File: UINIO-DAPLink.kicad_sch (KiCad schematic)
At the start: 44 parts, among them J1 扩展板串口 & 电源输出, J2 扩展板 JTAG 输出, J3 JTAG_nTRST 跳线选择, J4 3.3V 跳线选择, J5 扩展板 SWD 输入, J6 DAPLink 固件下载接口, J7 SWD 下载输出, U1 ME6211C33M5G, U2 STM32F103C8T6, Y1 8MHz

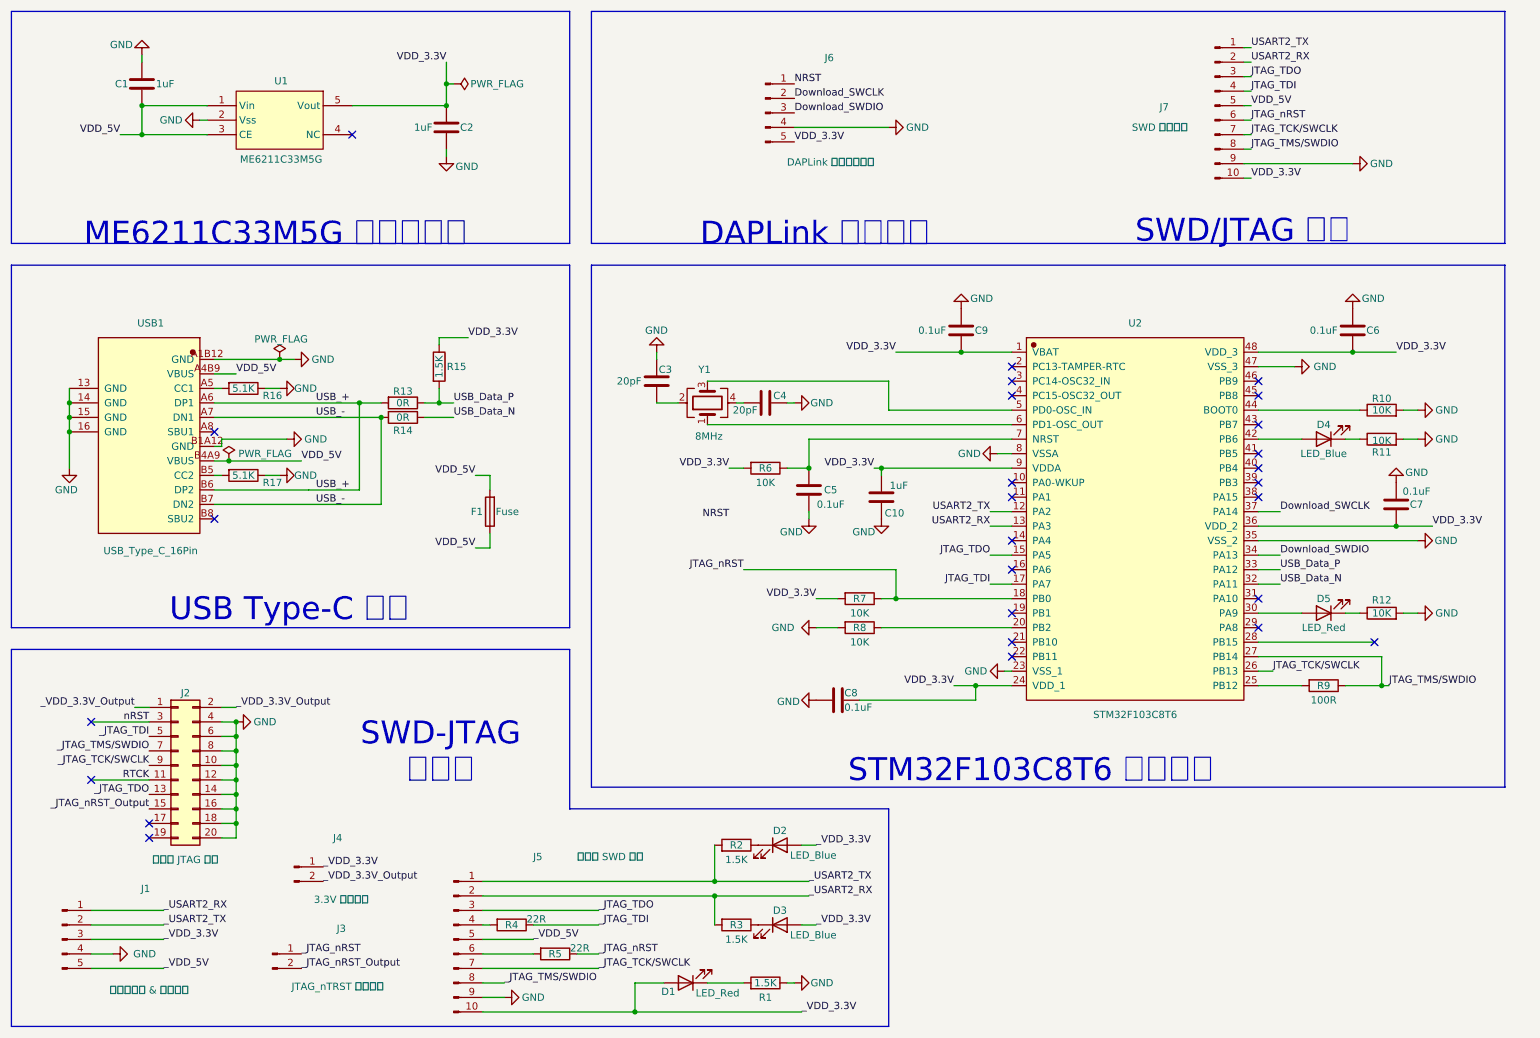
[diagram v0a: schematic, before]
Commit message: update
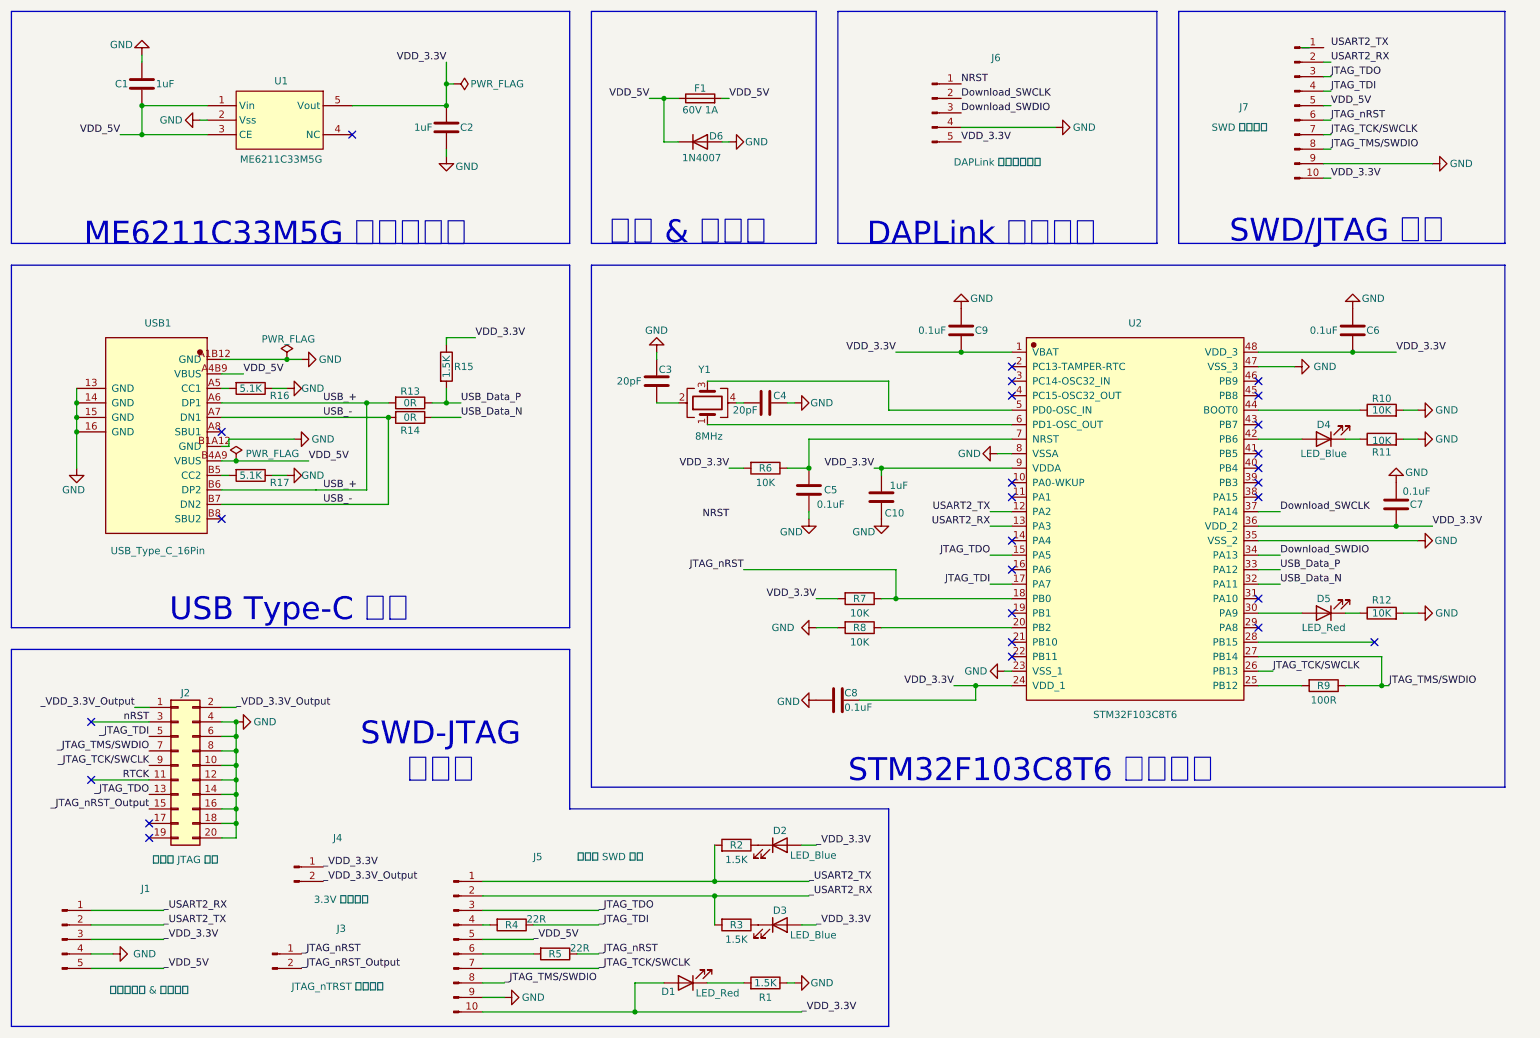
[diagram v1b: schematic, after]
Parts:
- added D6: 1N4007, Diode_THT:D_DO-41_SOD81_P10.16mm_Horizontal, symbol Diode:1N4007
- F1: value Fuse -> 60V 1A
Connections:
- net GND: now also D6.2 (A)
- net USART2_TX: no longer J7.1 (Pin_1)
- net VDD_5V: now also D6.1 (K)
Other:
- note added: "过流 & 防反接"
- moved on the sheet: F1, J6, J7, R13, R14, R15, R16, R17, USB1
